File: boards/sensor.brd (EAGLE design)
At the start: 20 x 20 mm, 18 parts

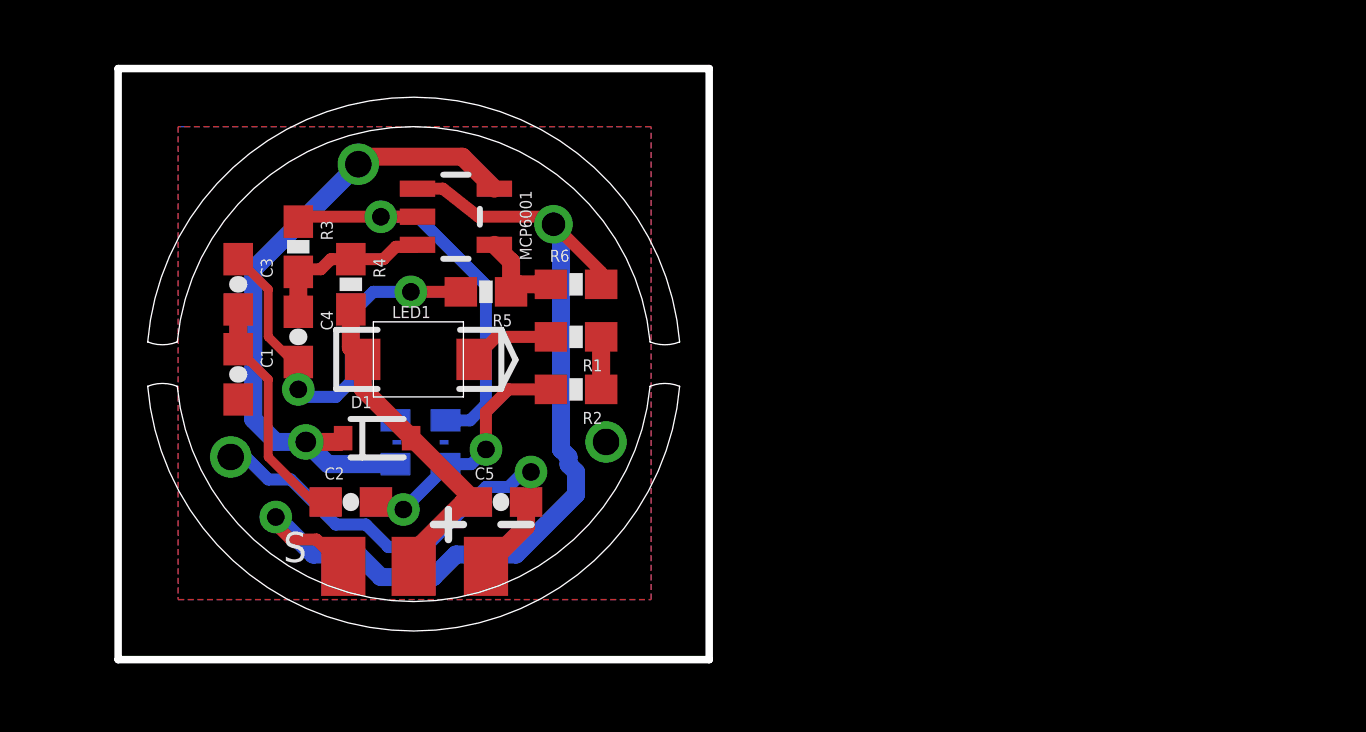
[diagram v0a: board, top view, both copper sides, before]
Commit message: put all the downloaded files into directories
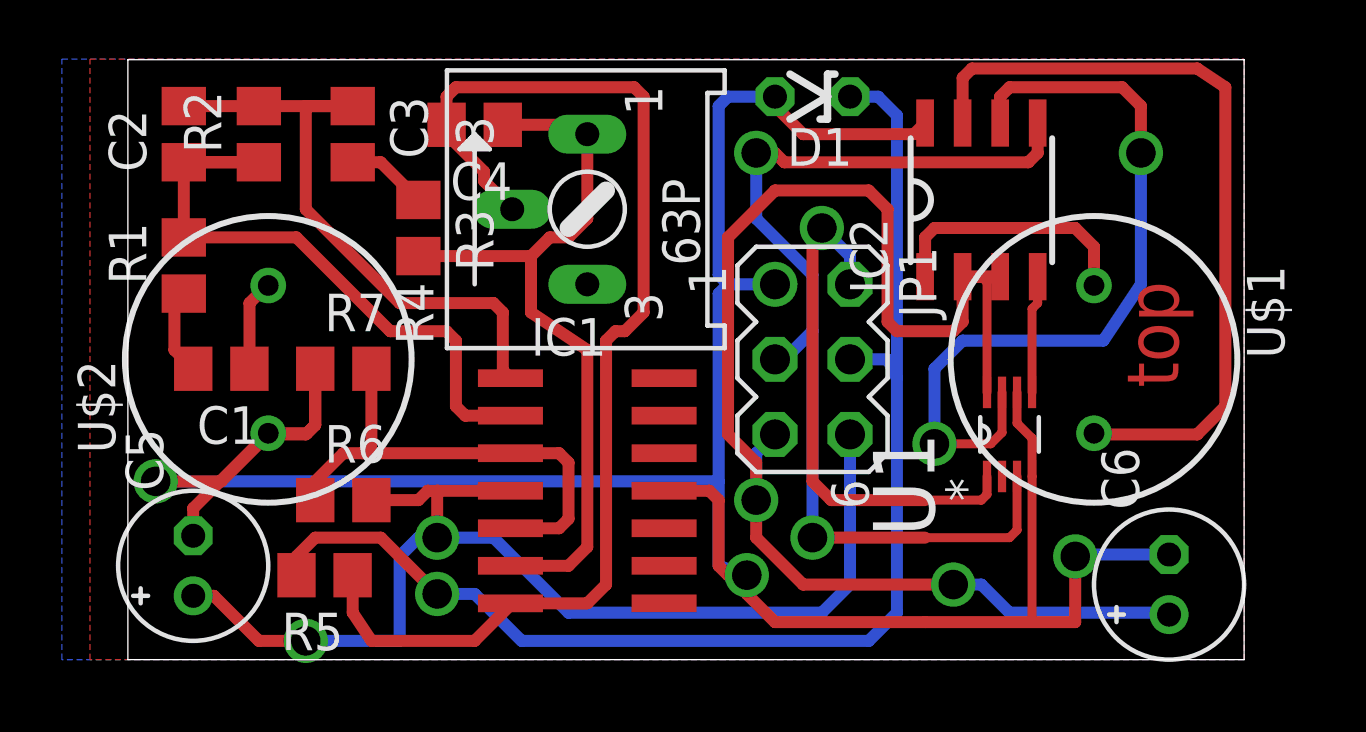
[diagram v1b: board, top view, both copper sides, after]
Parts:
- removed APDS1: (no value), librae:MINIATURE-CHIPLED
- removed GND, OUT, VCC: M01SMD-4.5X1.5, SparkFun-Connectors:PAD-1.5X4.5
- removed LED1: (no value), librae:LED-1206-REVERSE-MOUNT
- removed MCP6001: OPA344, SparkFun-AnalogIC:SOT23-5
- added C6: 10uF, rcl:E2-5
- added IC1: LM324D, linear:SO14
- added IC2: BD6211F, Ultrasound:SOP8
- added JP1: (no value), con-lstb:MA03-2
- added R7: 470, rcl:R0805
- added U$1, U$2: TRANSDUCER, Ultrasound:TRANSDUCER
- added U1: NC7NZ04K8X, Ultrasound:SOP50P310X90-8N
- C1: value 4.7uF -> 100n; device SparkFun-Capacitors:0603-CAP -> rcl:C0805
- C2, C3: value 4.7uF -> (none); device SparkFun-Capacitors:0603-CAP -> rcl:C0805
- C4: value 2.2uF -> (none); device SparkFun-Capacitors:0603-CAP -> rcl:C0805
- C5: value 2.2uF -> 10uF; device SparkFun-Capacitors:0603-CAP -> rcl:E2-5
- D1: value BAT20JFILM -> 3V3; device SparkFun-DiscreteSemi:SOD-323 -> diode:ZDIO-2.5
- R1: value 470 -> 1K5; device SparkFun-Resistors:0603-RES -> rcl:R0805
- R2: value 12K -> 5K6; device SparkFun-Resistors:0603-RES -> rcl:R0805
- R3: value 100K -> 1K5; device SparkFun-Resistors:0603-RES -> rcl:R0805
- R4: device SparkFun-Resistors:0603-RES -> pot:S63P
- R5: value 10K -> 100; device SparkFun-Resistors:0603-RES -> rcl:R0805
- R6: value 3.3M -> 1K; device SparkFun-Resistors:0603-RES -> rcl:R0805
- moved D1 18.7 mm to (23.5, 19.1), turned to 180 degrees
- moved R2 13.8 mm to (4.76, 17.8), turned to 90 degrees
- moved C2 13.7 mm to (2.22, 17.8), turned to 90 degrees
- moved R1 13.5 mm to (2.22, 13.3), turned to 90 degrees
- moved R5 11.0 mm to (6.99, 2.86)
- moved R6 10.7 mm to (7.62, 5.40)
- moved C5 10.6 mm to (2.54, 3.17), turned to 90 degrees
- moved C4 9.33 mm to (12.1, 18.1), turned to 180 degrees
- moved R4 8.39 mm to (15.9, 15.2), turned to 90 degrees
- moved C3 6.39 mm to (7.94, 17.8)
- moved R3 4.11 mm to (10.2, 14.6)
- moved C1 0.60 mm to (3.49, 9.84), turned to 180 degrees
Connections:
- removed net N$8: C1.1, C2.1, C3.2
- removed net OUT: MCP6001.1, OUT.P$1, R6.2
- removed net VCC: C5.1, D1.2, LED1.A, R4.2, VCC.P$1
- removed net VDD: APDS1.P$1, D1.1, MCP6001.5
- new net N$1: C2.1, IC1.2, R1.2, R2.1
- new net N$11: IC2.7, U$1.2
- new net N$12: IC2.6, U1.7
- new net N$13: IC2.4, U1.5
- new net N$2: C1.2, R1.1
- new net N$5: C3.2, R3.1
- new net REF: IC1.3, IC1.5, R6.1, R7.2
- new net RX: D1.C, JP1.4, R5.2
- new net RXP: C5.+, IC1.4, JP1.6, R6.2
- new net TX: IC2.5, JP1.3, U1.3
- new net TXP: C6.+, IC2.2, IC2.3, JP1.5, U1.8
- new net TX_EN: JP1.2, U1.1
- net GND: now also C5.-, C6.-, D1.A, IC1.11, IC2.8, JP1.1, R7.1, U$2.1, U1.4, U1.6; no longer APDS1.P$4, C1.2, C5.2, GND.P$1, MCP6001.2, R1.1, R2.1, R3.1
- net N$10: now also IC2.1, U$1.1; no longer C4.1, MCP6001.3, R3.2, R4.1
- net N$3: now also C2.2, C3.1, IC1.1, R2.2; no longer LED1.C, R1.2
- net N$6: now also C4.1, IC1.6, R3.2, R4.A; no longer MCP6001.4, R5.1, R6.1
- net N$7: now also C4.2, IC1.7, R4.S, R5.1; no longer APDS1.P$6, C2.2, R2.2
- net N$9: now also C1.1, U$2.2; no longer C3.1, C4.2, R5.2
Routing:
- net GND: track 32.6 -> 96.0 mm, vias 4 -> 3
- net TXP: track 0.00 -> 49.3 mm, vias 0 -> 2
- net RX: track 0.00 -> 43.7 mm, vias 0 -> 1
- net RXP: track 0.00 -> 38.9 mm, vias 0 -> 2
- net TX: track 0.00 -> 35.1 mm, vias 0 -> 2
- net OUT: track 32.5 -> 0.00 mm, vias 2 -> 0
- net N$7: track 8.66 -> 40.4 mm, vias 2 -> 0
- net N$12: track 0.00 -> 26.8 mm, vias 0 -> 2
- net N$11: track 0.00 -> 26.4 mm
- net N$6: track 3.28 -> 25.8 mm
- net N$1: track 0.00 -> 22.5 mm
- net VDD: track 22.0 -> 0.00 mm, vias 2 -> 0
- net N$3: track 2.92 -> 21.2 mm
- net TX_EN: track 0.00 -> 17.9 mm, vias 0 -> 1
- net REF: track 0.00 -> 16.7 mm
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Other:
- board size 20 x 20 mm -> 37.8 x 20.3 mm
- board text added: "top"
- board text removed: "APDS1"
- board text removed: "C1"
- board text removed: "C2"
- board text removed: "C3"
- board text removed: "C4"
- board text removed: "C5"
- board text removed: "JP1"
- board text removed: "LED1"
- board text removed: "MCP6001"
- board text removed: "R1"
- board text removed: "R2"
- board text removed: "R3"
- board text removed: "R4"
- board text removed: "R5"
- board text removed: "R6"
- board text removed: "S"
- board text removed: "SCHOTTKEY"
